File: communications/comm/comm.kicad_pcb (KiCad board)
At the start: 2 copper layers, 37.9 x 36.7 mm, 1 part, among them J1 Conn_Coaxial

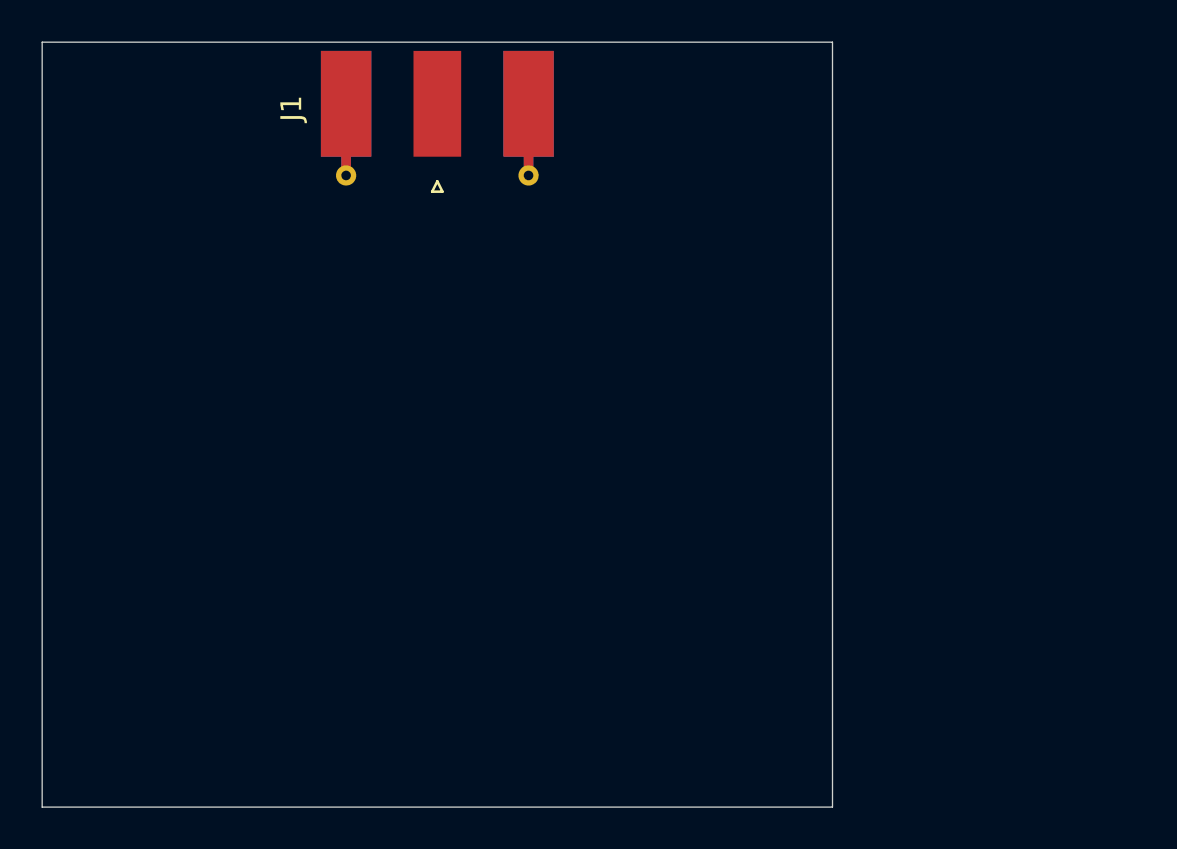
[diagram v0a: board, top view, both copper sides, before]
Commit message: refresh
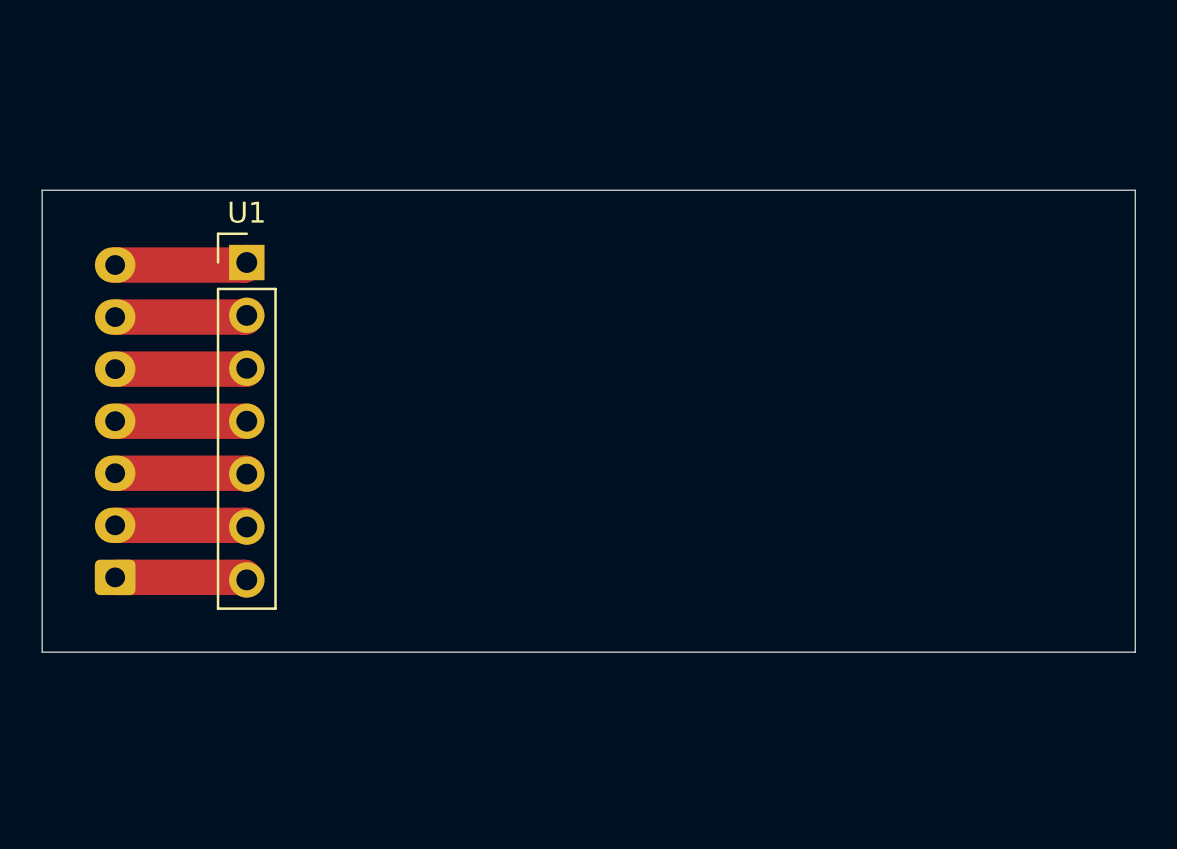
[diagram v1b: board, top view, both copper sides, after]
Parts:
- added U1: SX1276, Connector_PinHeader_2.54mm:PinHeader_1x07_P2.54mm_Vertical, F.Cu at (142.2, 80.7)
- J1: value Conn_Coaxial -> Screw_Terminal_01x07; footprint Connector_Coaxial:SMA_Molex_73251-1153_EdgeMount_Horizontal -> Connector_JST:JST_EH_B7B-EH-A_1x07_P2.50mm_Vertical; moved to B.Cu
- moved J1 26.1 mm to (135.9, 95.8), turned to 90 degrees
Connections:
- J1 pad 1: unconnected-(J1-In-Pad1) -> Net-(J1-Pin_1)
- J1 pad 2: unconnected-(J1-Ext-Pad2) -> Net-(J1-Pin_2)
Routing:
- net Net-(J1-Pin_7): track 0.00 -> 6.37 mm
- net Net-(J1-Pin_1): track 0.00 -> 6.37 mm
- net Net-(J1-Pin_6): track 0.00 -> 6.35 mm
- net Net-(J1-Pin_2): track 0.00 -> 6.35 mm
- net Net-(J1-Pin_3): track 0.00 -> 6.34 mm
- net Net-(J1-Pin_5): track 0.00 -> 6.34 mm
- net Net-(J1-Pin_4): track 0.00 -> 6.32 mm
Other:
- board size 37.9 x 36.7 mm -> 52.5 x 22.2 mm
